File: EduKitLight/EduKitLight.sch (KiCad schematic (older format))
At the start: 7 parts, among them P1 CONN_01X05, P2 CONN_01X04, P3 CONN_01X02, P5 CONN_01X05, U1 uln2803A, U2 Arduino_Mini

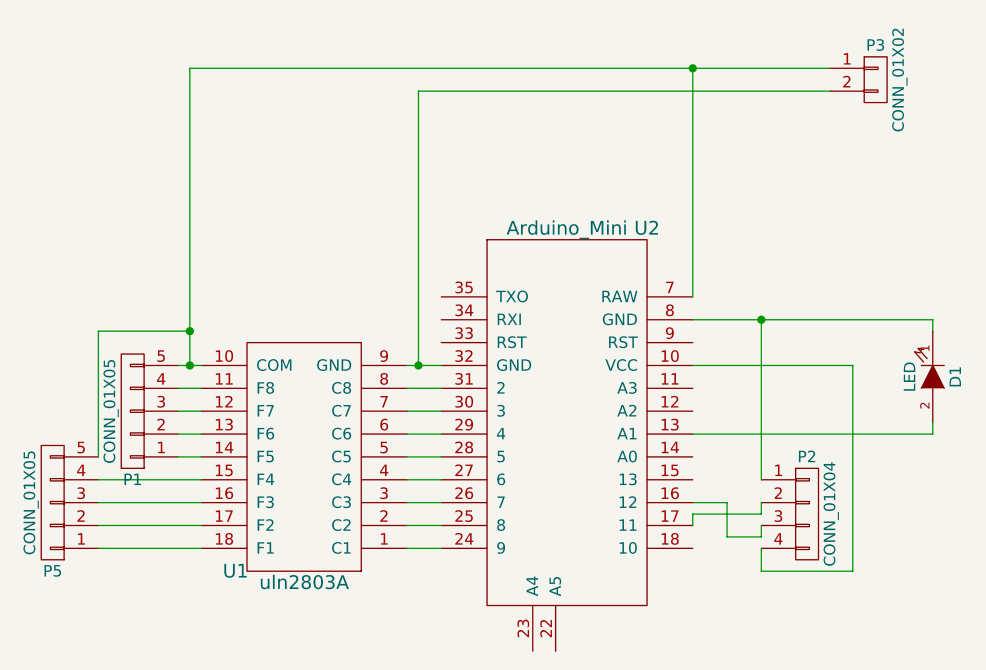
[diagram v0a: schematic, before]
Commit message: Full reafactored, v 1.1
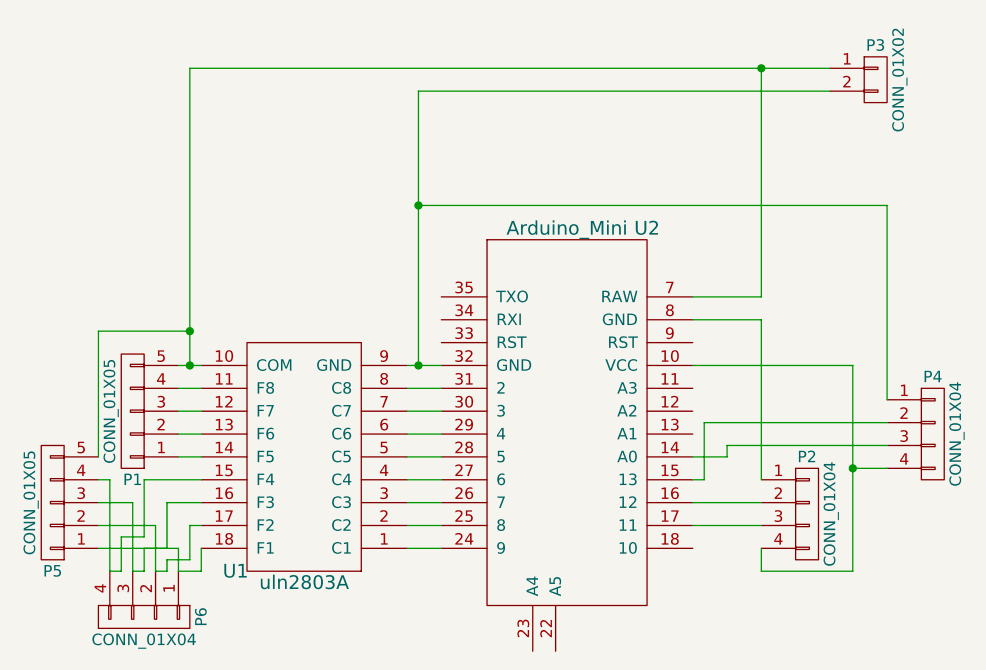
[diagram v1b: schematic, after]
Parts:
- removed D1: LED, LEDs:LED-5MM, symbol LED
- added P4, P6: CONN_01X04, Pin_Headers:Pin_Header_Straight_1x04, symbol CONN_01X04
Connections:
- net at P2.4 (P4), U2.10 (VCC): now also P4.4 (P4)
- net at U2.14 (A0): now also P4.3 (P3)
- net at U2.15 (13): now also P4.2 (P2)
- net at U2.16 (12): now also P2.2 (P2); no longer P2.3 (P3)
- net at U2.17 (11): now also P2.3 (P3); no longer P2.2 (P2)
- net at P3.2 (P2), U1.9 (GND), U2.32 (GND): now also P4.1 (P1)
- net at P5.4 (P4), U1.15 (F4): now also P6.4 (P4)
- net at P5.3 (P3), U1.16 (F3): now also P5.1 (P1), U1.18 (F1), P6.1 (P1), P6.3 (P3)
- net at P5.2 (P2), U1.17 (F2): now also P6.2 (P2)
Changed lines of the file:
@@
 LIBS:valves
 LIBS:bugs
-LIBS:bug-cache
+LIBS:EduKitLight-cache
 EELAYER 25 0
 EELAYER END
@@
 	-1   0    0    1
 $EndComp
-Wire Wire Line
-	4300 3850 4150 3850
-Wire Wire Line
-	4150 3950 4300 3950
-Wire Wire Line
-	4300 4150 4150 4150
-Wire Wire Line
-	5400 2050 5400 3050
-Wire Wire Line
-	3150 3350 3250 3350
-Wire Wire Line
-	3150 3450 3250 3450
-Wire Wire Line
-	3150 3550 3250 3550
-Wire Wire Line
-	3150 3650 3250 3650
-Wire Wire Line
-	3150 3750 3250 3750
-Wire Wire Line
-	2800 3850 3250 3850
-Wire Wire Line
-	2800 3950 3250 3950
-Wire Wire Line
-	2800 4050 3250 4050
-Wire Wire Line
-	2800 4150 3250 4150
-Wire Wire Line
-	4300 4050 4150 4050
-Wire Wire Line
-	4150 3750 4300 3750
-Wire Wire Line
-	4300 3650 4150 3650
-Wire Wire Line
-	4150 3550 4300 3550
-Wire Wire Line
-	4300 3450 4150 3450
-Connection ~ 3200 3350
-Wire Wire Line
-	4150 3350 4300 3350
-Connection ~ 3200 3200
-Wire Wire Line
-	2800 3750 2800 3200
-Wire Wire Line
-	2800 3200 3200 3200
-Wire Wire Line
-	4200 2150 6000 2150
-Wire Wire Line
-	3200 2050 3200 3350
-Connection ~ 5400 2050
-Wire Wire Line
-	3200 2050 6000 2050
-Wire Wire Line
-	4200 2150 4200 3350
-Connection ~ 4200 3350
-Wire Wire Line
-	5700 4250 5700 4150
-Wire Wire Line
-	5400 3350 6100 3350
 $Comp
 L CONN_01X02 P3
@@
 	1    0    0    -1
 $EndComp
+$Comp
+L CONN_01X04 P4
+U 1 1 5899E550
+P 6450 3650
+F 0 "P4" H 6450 3900 50  0000 C CNN
+F 1 "CONN_01X04" V 6550 3650 50  0000 C CNN
+F 2 "Pin_Headers:Pin_Header_Straight_1x04" H 6450 3650 50  0001 C CNN
+F 3 "" H 6450 3650 50  0000 C CNN
+	1    6450 3650
+	1    0    0    -1
+$EndComp
+$Comp
+L CONN_01X04 P6
+U 1 1 5899F62E
+P 3000 4450
+F 0 "P6" H 3000 4700 50  0000 C CNN
+F 1 "CONN_01X04" V 3100 4450 50  0000 C CNN
+F 2 "Pin_Headers:Pin_Header_Straight_1x04" H 3000 4450 50  0001 C CNN
+F 3 "" H 3000 4450 50  0000 C CNN
+	1    3000 4450
+	0    1    1    0
+$EndComp
+Wire Wire Line
+	4300 3850 4150 3850
+Wire Wire Line
+	4150 3950 4300 3950
+Wire Wire Line
+	4300 4150 4150 4150
+Wire Wire Line
+	3150 3350 3250 3350
+Wire Wire Line
+	3150 3450 3250 3450
+Wire Wire Line
+	3150 3550 3250 3550
+Wire Wire Line
+	3150 3650 3250 3650
+Wire Wire Line
+	3150 3750 3250 3750
+Wire Wire Line
+	4300 4050 4150 4050
+Wire Wire Line
+	4150 3750 4300 3750
+Wire Wire Line
+	4300 3650 4150 3650
+Wire Wire Line
+	4150 3550 4300 3550
+Wire Wire Line
+	4300 3450 4150 3450
+Connection ~ 3200 3350
+Wire Wire Line
+	4150 3350 4300 3350
+Connection ~ 3200 3200
+Wire Wire Line
+	2800 3750 2800 3200
+Wire Wire Line
+	2800 3200 3200 3200
+Wire Wire Line
+	4200 2150 6000 2150
+Wire Wire Line
+	3200 2050 3200 3350
+Wire Wire Line
+	3200 2050 6000 2050
+Wire Wire Line
+	4200 2150 4200 3350
+Connection ~ 4200 3350
+Wire Wire Line
+	5700 4250 5700 4150
+Wire Wire Line
+	5400 3350 6100 3350
+Wire Wire Line
+	6100 4250 5700 4250
+Wire Wire Line
+	5700 3850 5700 3150
+Wire Wire Line
+	5700 3050 5400 3050
+Wire Wire Line
+	5700 3050 5700 2050
+Connection ~ 5700 2050
+Wire Wire Line
+	5700 3150 5400 3150
+Wire Wire Line
+	6250 3500 6250 2650
+Wire Wire Line
+	6250 2650 4200 2650
+Connection ~ 4200 2650
+Wire Wire Line
+	6250 3800 6100 3800
+Connection ~ 6100 3800
+Wire Wire Line
+	5700 4050 5400 4050
+Wire Wire Line
+	5700 3950 5400 3950
 Wire Wire Line
 	6100 3350 6100 4250
 Wire Wire Line
-	6100 4250 5700 4250
-Wire Wire Line
-	5700 3850 5700 3150
-Wire Wire Line
-	5400 3150 6450 3150
-Wire Wire Line
-	5550 4100 5700 4100
-Wire Wire Line
-	5700 4100 5700 4050
-Wire Wire Line
-	5700 3950 5700 4000
-Wire Wire Line
-	5700 4000 5400 4000
-Wire Wire Line
-	5400 4000 5400 4050
-Wire Wire Line
-	5400 3950 5550 3950
-Wire Wire Line
-	5550 3950 5550 4100
-$Comp
-L LED D1
-U 1 1 5894CBA6
-P 6450 3400
-F 0 "D1" H 6450 3500 50  0000 C CNN
-F 1 "LED" H 6450 3300 50  0000 C CNN
-F 2 "LEDs:LED-5MM" H 6450 3400 50  0001 C CNN
-F 3 "" H 6450 3400 50  0000 C CNN
-	1    6450 3400
-	0    1    1    0
-$EndComp
-Wire Wire Line
-	6450 3150 6450 3200
-Connection ~ 5700 3150
-Wire Wire Line
-	5400 3650 6450 3650
-Wire Wire Line
-	6450 3650 6450 3600
+	6250 3600 5450 3600
+Wire Wire Line
+	5550 3700 6250 3700
+Wire Wire Line
+	5550 3750 5400 3750
+Wire Wire Line
+	5550 3750 5550 3700
+Wire Wire Line
+	5450 3600 5450 3850
+Wire Wire Line
+	5450 3850 5400 3850
+Wire Wire Line
+	3250 4150 3250 4250
+Wire Wire Line
+	3250 4250 3150 4250
+Wire Wire Line
+	3250 4050 3200 4050
+Wire Wire Line
+	3200 4050 3200 4200
+Wire Wire Line
+	3200 4200 3100 4200
+Wire Wire Line
+	3100 4200 3100 4250
+Wire Wire Line
+	3100 4250 3050 4250
+Wire Wire Line
+	3250 3950 3100 3950
+Wire Wire Line
+	3100 3950 3100 4150
+Wire Wire Line
+	3100 4150 3000 4150
+Wire Wire Line
+	3000 4150 3000 4250
+Wire Wire Line
+	3000 4250 2950 4250
+Wire Wire Line
+	3250 3850 3000 3850
+Wire Wire Line
+	3000 3850 3000 4100
+Wire Wire Line
+	3000 4100 2900 4100
+Wire Wire Line
+	2900 4100 2900 4250
+Wire Wire Line
+	2900 4250 2850 4250
+Wire Wire Line
+	2800 4150 3150 4150
+Wire Wire Line
+	3150 4150 3150 4250
+Wire Wire Line
+	2800 4050 3050 4050
+Wire Wire Line
+	3050 4050 3050 4250
+Wire Wire Line
+	2800 3950 2950 3950
+Wire Wire Line
+	2950 3950 2950 4250
+Wire Wire Line
+	2800 3850 2850 3850
+Wire Wire Line
+	2850 3850 2850 4250
 $EndSCHEMATC
